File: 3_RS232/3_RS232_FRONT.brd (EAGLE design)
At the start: 71.5 x 24 mm, 1 part

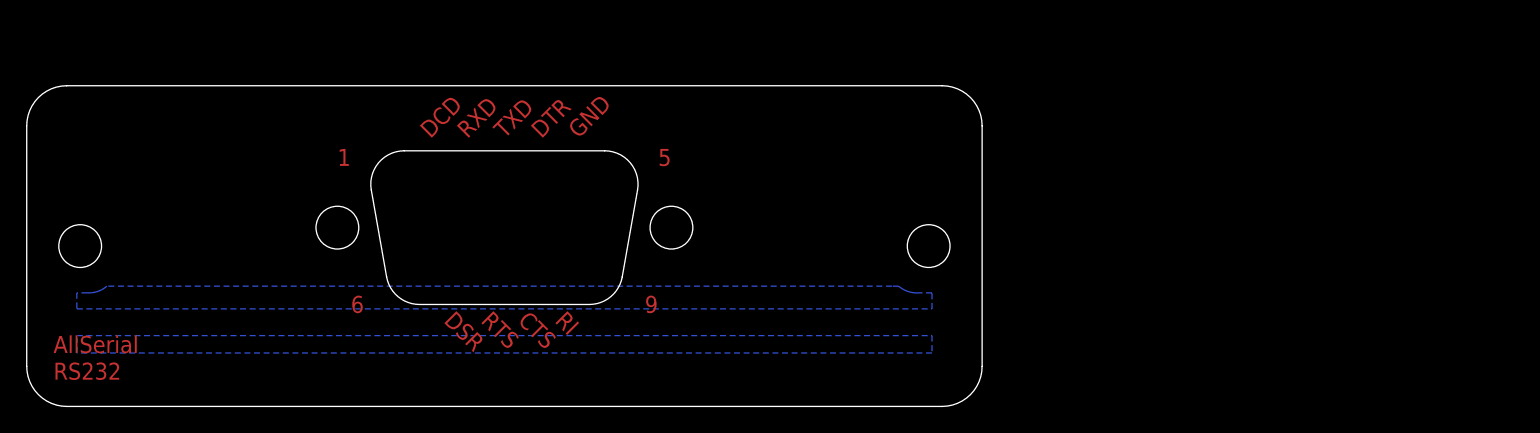
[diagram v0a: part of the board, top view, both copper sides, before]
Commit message: Cleanup, front with lib elements
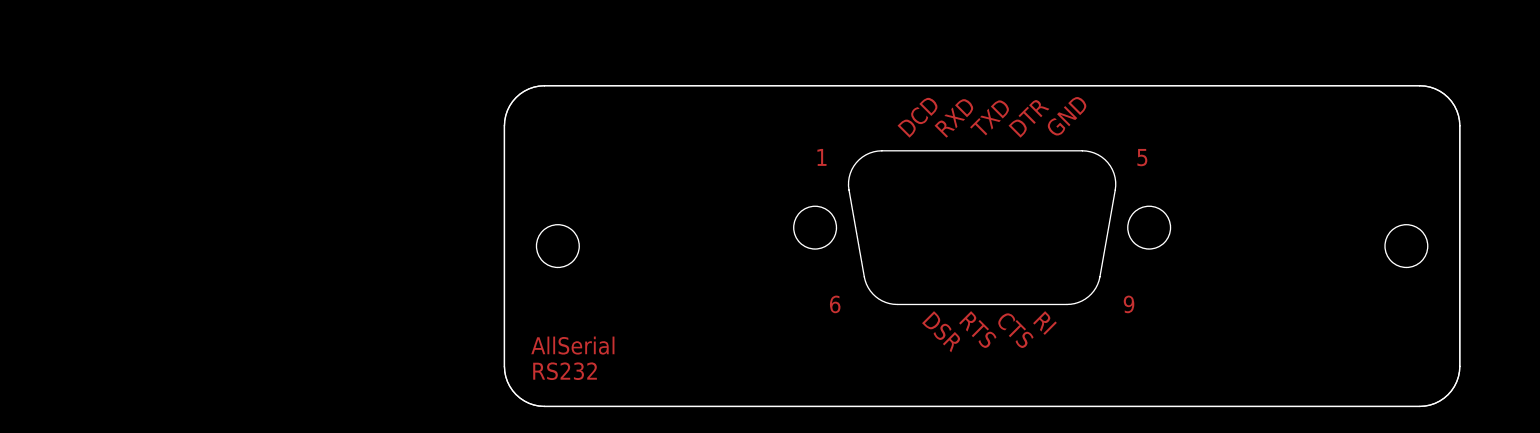
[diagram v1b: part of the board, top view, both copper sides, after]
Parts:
- removed E$1: (no value), AllSerialv2:PANEL
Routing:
- removed copper zone on layer 16, net S$1
- removed copper zone on layer 16, net S$2
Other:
- outline, holes or cut-outs redrawn
- board text added: "AllSerial RS232"
- board text removed: "RS232"
